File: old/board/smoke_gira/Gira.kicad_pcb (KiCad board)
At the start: 2 copper layers, 38 x 53.2 mm, 14 parts, among them J1 Moat_Bus_wire, J2 1wireConn, J3 I2C, J4 Conn_01x06

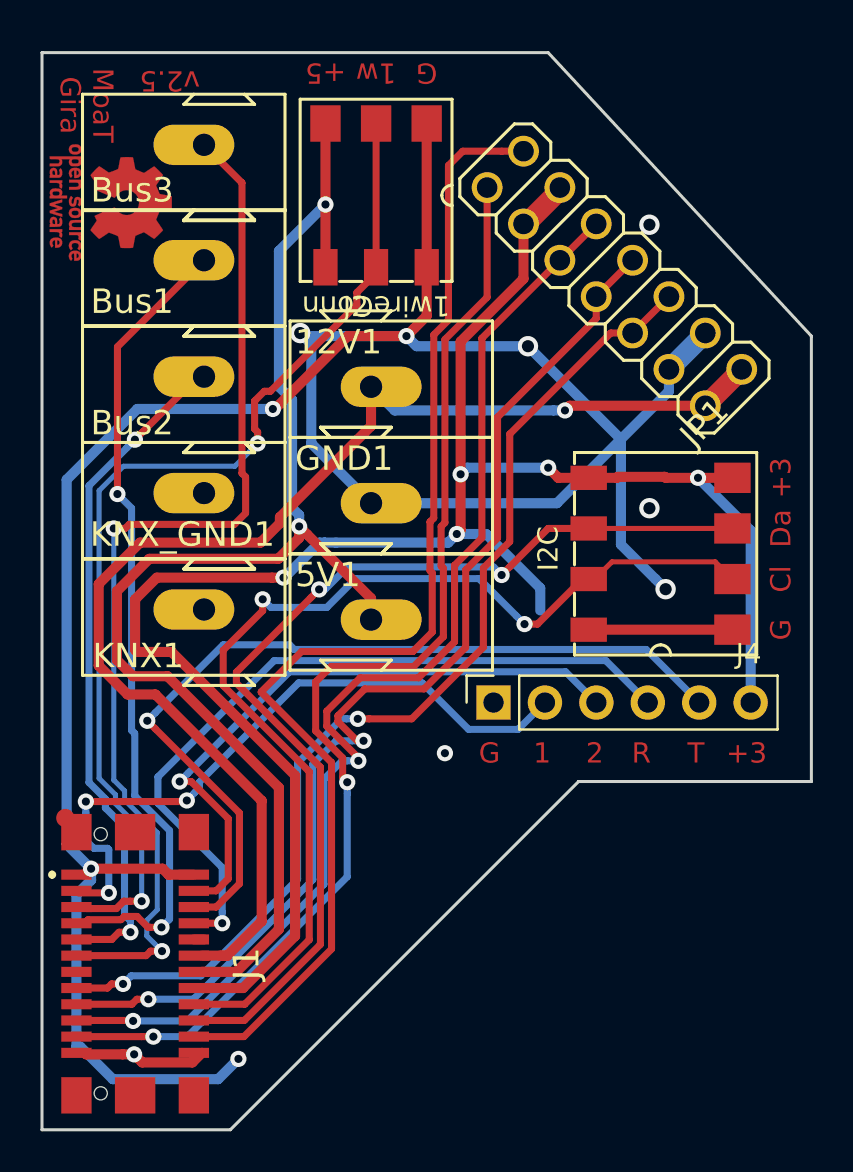
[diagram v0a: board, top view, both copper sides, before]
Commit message: updated
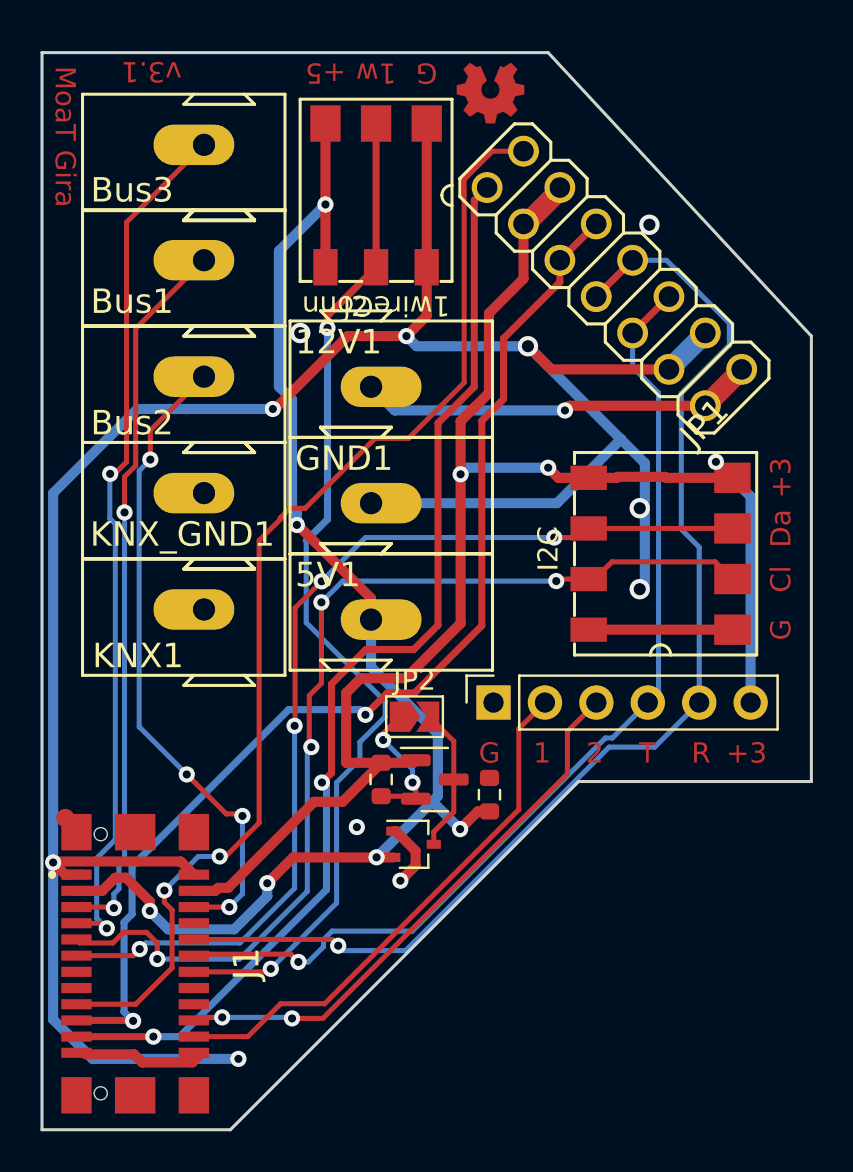
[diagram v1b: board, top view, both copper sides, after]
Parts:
- removed REF**: OSHW-Logo_5.7x6mm_Copper, Symbol:OSHW-Logo_5.7x6mm_Copper
- added D1: BAT54SW, Package_TO_SOT_SMD:SOT-323_SC-70, F.Cu at (147.8, 111.6)
- added G***: LOGO, localstuff:OSHW Logo 3mm Cu, F.Cu at (151.7, 74.5)
- added JP2: SolderJumper_2_Open, Jumper:SolderJumper-2_P1.3mm_Open_TrianglePad1.0x1.5mm, F.Cu at (147.9, 105.3)
- added Q1: 2N7002, Package_TO_SOT_SMD:SOT-23, F.Cu at (148.9, 108.4)
- added R1: 10k, Resistor_SMD:R_0603_1608Metric, F.Cu at (146.2, 108.4)
- added R2: 10k, Resistor_SMD:R_0603_1608Metric, F.Cu at (151.6, 109.2)
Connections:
- Bus1 pad 1: Net-(Bus1-Pad1) -> Net-(Bus1-Pin_1)
- Bus2 pad 1: Net-(Bus2-Pad1) -> Net-(Bus2-Pin_1)
- Bus3 pad 1: Net-(Bus3-Pad1) -> Net-(J1-Bus_3)
- J1 pad 10: +12V -> /RxD
- J1 pad 11: Net-(Bus3-Pad1) -> /SDA
- J1 pad 12: +12V -> /TxD
- J1 pad 13: (no net) -> unconnected-(J1-S5)
- J1 pad 14: +5V -> /1wire
- J1 pad 15: /TxD -> unconnected-(J1-S4)
- J1 pad 16: +3V3 -> unconnected-(J1-T4)
- J1 pad 17: /RxD -> /Unk_2
- J1 pad 18: /SCL -> unconnected-(J1-T3)
- J1 pad 20: /SDA -> /T2
- J1 pad 22: /Unk_2 -> /T1
- J1 pad 3: Net-(J1-Pad3) -> +5V
- J1 pad 4: Net-(J1-Pad4) -> +3V3
- J1 pad 5: /1wire -> Net-(Bus1-Pin_1)
- J1 pad 6: Net-(J1-Pad6) -> Net-(Bus2-Pin_1)
- J1 pad 7: Net-(Bus1-Pad1) -> Net-(J1-Bus_3)
- J1 pad 8: Net-(J1-Pad8) -> unconnected-(J1-Bus_4)
- J1 pad 9: Net-(Bus2-Pad1) -> /SCL
- J4 pad 2: Net-(J1-Pad3) -> /T1
- J4 pad 3: Net-(J1-Pad4) -> /T2
- J4 pad 4: Net-(J1-Pad8) -> /TxD
- J4 pad 5: Net-(J1-Pad6) -> /RxD
- KNX1 pad 1: (no net) -> unconnected-(KNX1-Pin_1)
- KNX_GND1 pad 1: (no net) -> unconnected-(KNX_GND1-Pin_1)
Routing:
- net Net-(Bus3-Pad1): track 52.1 -> 0.00 mm, vias 2 -> 0
- net +12V: track 63.7 -> 19.6 mm
- net Net-(J1-Bus_3): track 0.00 -> 43.1 mm, vias 0 -> 2
- net Net-(J1-Pad6): track 42.7 -> 0.00 mm, vias 1 -> 0
- net Net-(Bus1-Pad1): track 40.1 -> 0.00 mm, vias 2 -> 0
- net Net-(J1-Pad8): track 37.4 -> 0.00 mm, vias 1 -> 0
- net Net-(Bus1-Pin_1): track 0.00 -> 35.7 mm, vias 0 -> 2
- net Net-(J1-Pad3): track 33.8 -> 0.00 mm, vias 3 -> 0
- net Net-(Bus2-Pad1): track 33.2 -> 0.00 mm, vias 2 -> 0
- net Net-(Bus2-Pin_1): track 0.00 -> 32.1 mm, vias 0 -> 4
- net Net-(J1-Pad4): track 31.5 -> 0.00 mm, vias 1 -> 0
- net /T2: track 0.00 -> 27.6 mm, vias 0 -> 2
- net /T1: track 0.00 -> 26.5 mm
- net +3V3: track 95.4 -> 75.9 mm, vias 5 -> 3
- net /1wire_5: track 0.00 -> 7.21 mm
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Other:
- net class Default removed
- net class Power removed
- board text added: "v3.1"
- board text removed: "v2.5"
